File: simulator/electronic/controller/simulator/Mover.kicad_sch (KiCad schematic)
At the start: 4 parts, among them U2 STSPIN220

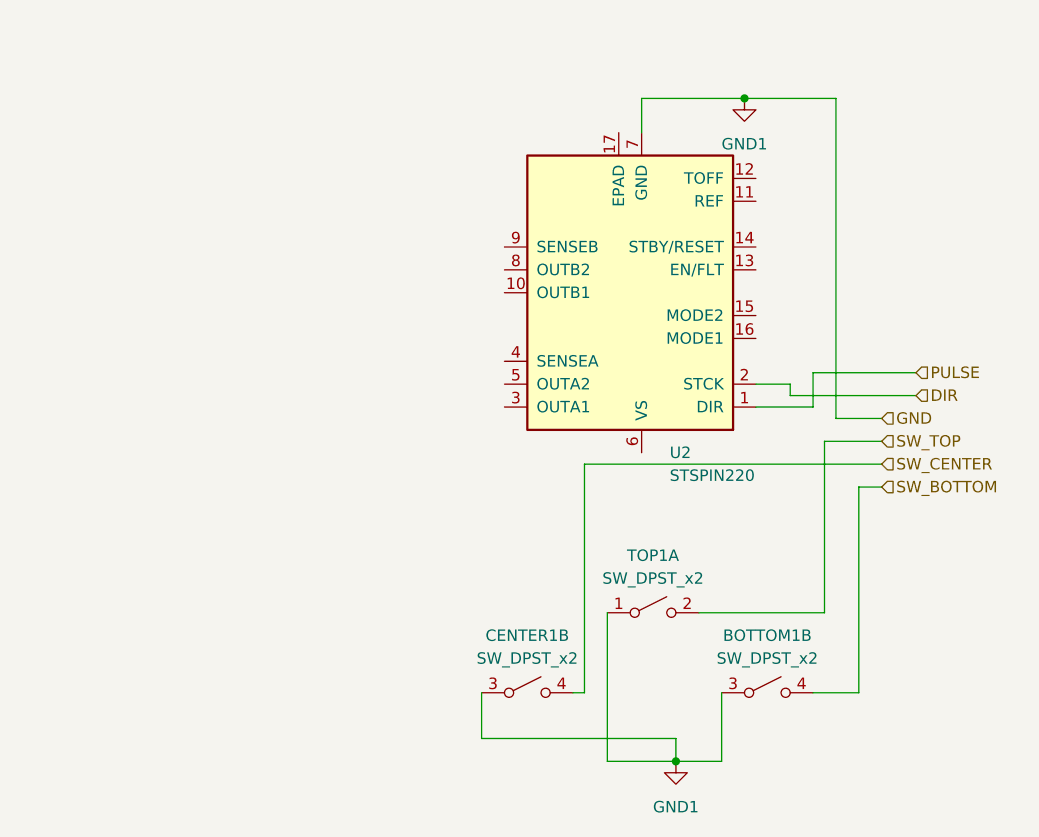
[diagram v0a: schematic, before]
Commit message: finalized schematics and PCB
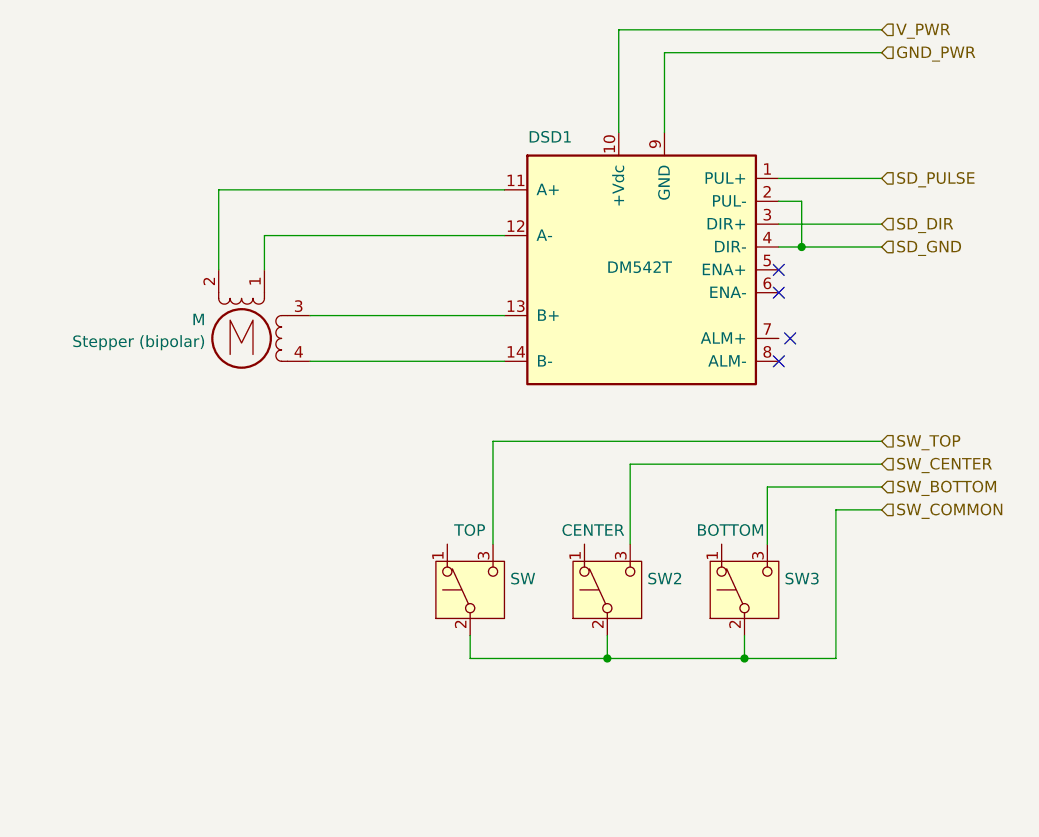
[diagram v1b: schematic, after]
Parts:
- removed BOTTOM1, CENTER1, TOP1: SW_DPST_x2, symbol Switch:SW_DPST_x2
- removed U2: STSPIN220, Package_DFN_QFN:VQFN-16-1EP_3x3mm_P0.5mm_EP1.8x1.8mm, symbol Driver_Motor:STSPIN220
- added DSD1: DM542T, symbol UO_Electrical_Components:DM542T
- added M: Stepper (bipolar), symbol Motor:Stepper_Motor_bipolar
- added SW: TOP, symbol Switch:SW_Push_SPDT
- added SW2: CENTER, symbol Switch:SW_Push_SPDT
- added SW3: BOTTOM, symbol Switch:SW_Push_SPDT
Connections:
- net SW_BOTTOM: now also SW3.3 (C)
- net SW_CENTER: now also SW2.3 (C)
- net SW_TOP: now also SW.3 (C)
- new net: DSD1.12 (A-), M.1
- new net: DSD1.11 (A+), M.2 (-)
- new net: DSD1.13 (B+), M.3
- new net: DSD1.14 (B-), M.4
- new net GND_PWR: DSD1.9 (GND)
- new net SD_DIR: DSD1.3 (DIR+)
- new net SD_GND: DSD1.2 (PUL-), DSD1.4 (DIR-)
- new net SD_PULSE: DSD1.1 (PUL+)
- new net SW_COMMON: SW.2 (B), SW2.2 (B), SW3.2 (B)
- new net V_PWR: DSD1.10 (+Vdc)
- no-connect marks 0 -> 4
